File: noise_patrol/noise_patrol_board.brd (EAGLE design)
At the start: 53.5 x 57.3 mm, 25 parts, among them IC1 4511D, Q1 TIP31C, U1 OPA345NA/3K

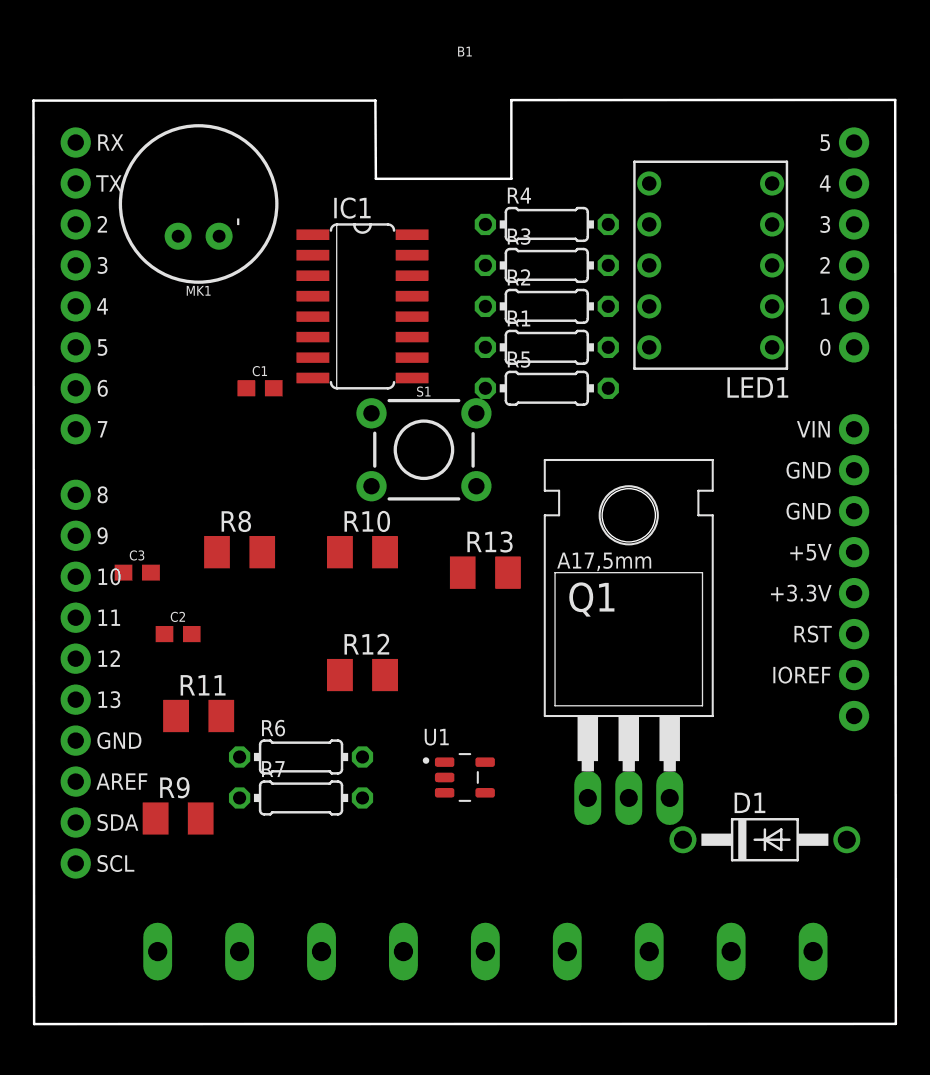
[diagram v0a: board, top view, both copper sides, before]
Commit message: Finished
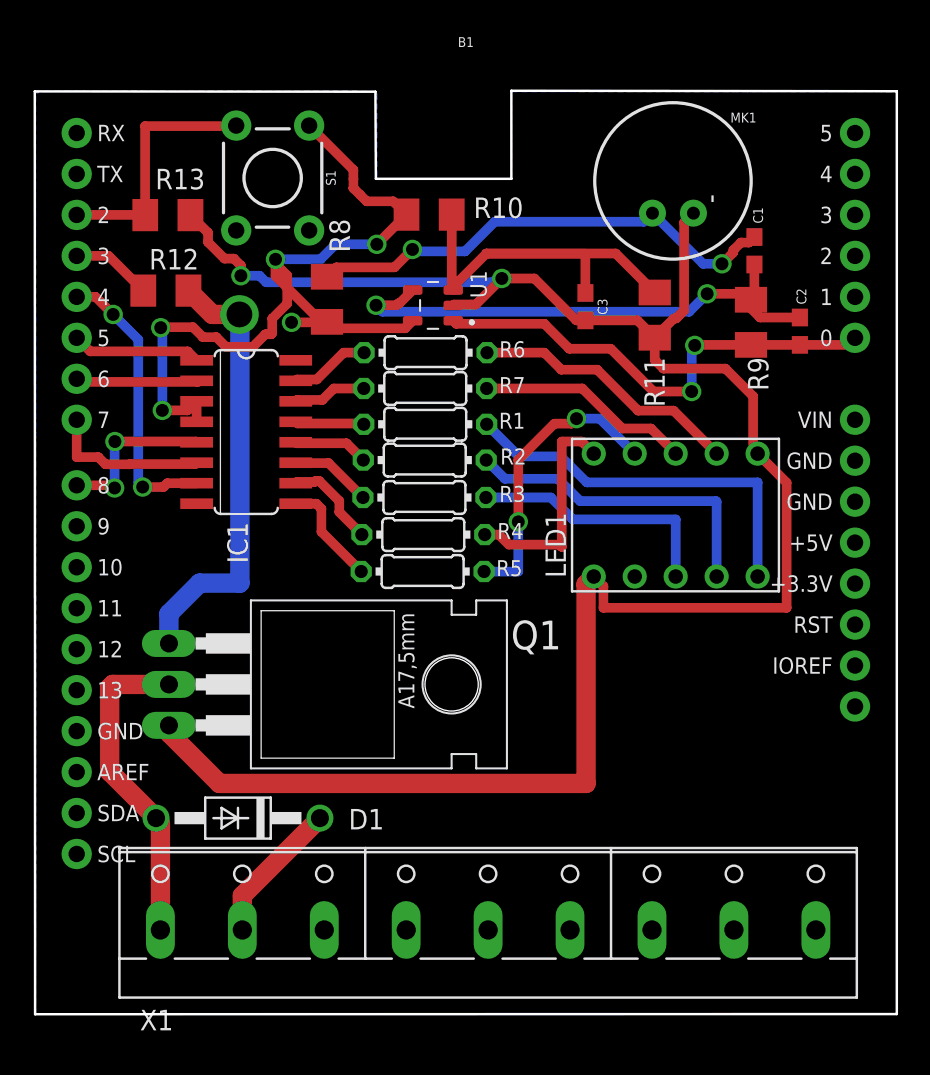
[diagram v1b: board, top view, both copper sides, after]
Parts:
- S1: value MOMENTARY-SWITCH-SPST-PTH-6.0MM -> Reset button
- moved R9 47.0 mm to (63.5, 58.7), turned to 270 degrees
- moved C2 42.9 mm to (66.5, 58.1), turned to 270 degrees
- moved R11 37.7 mm to (57.5, 59.1), turned to 270 degrees
- moved D1 32.7 mm to (31.6, 28.0), turned to 180 degrees
- moved C3 32.3 mm to (53.2, 59.7), turned to 270 degrees
- moved C1 31.8 mm to (63.7, 63.1), turned to 270 degrees
- moved R13 29.7 mm to (27.3, 65.3), turned to 180 degrees
- moved MK1 29.4 mm to (58.6, 67.5)
- moved U1 29.3 mm to (43.7, 59.8), turned to 180 degrees
- moved R12 26.8 mm to (27.2, 60.7)
- moved R7 26.5 mm to (43.3, 54.6)
- moved R6 26.2 mm to (43.3, 56.8)
- moved Q1 22.2 mm to (33.7, 36.2), turned to 270 degrees
- moved R10 21.3 mm to (43.5, 65.4)
- moved R4 20.7 mm to (43.1, 45.5)
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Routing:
- net GND: track 0.00 -> 121.9 mm, vias 0 -> 2
- net 5V: track 0.00 -> 53.8 mm, vias 0 -> 5
- net N$21: track 0.00 -> 32.8 mm, vias 0 -> 2
- net N$20: track 0.00 -> 30.3 mm, vias 0 -> 2
- net N$18: track 0.00 -> 29.7 mm, vias 0 -> 2
- net N$24: track 0.00 -> 27.7 mm
- net N$23: track 0.00 -> 27.5 mm, vias 0 -> 1
- net N$13: track 0.00 -> 24.1 mm
- net N$25: track 0.00 -> 20.1 mm
- net N$12: track 0.00 -> 20.0 mm
- net N$9: track 0.00 -> 18.2 mm, vias 0 -> 2
- net N$14: track 0.00 -> 17.6 mm, vias 0 -> 2
- net N$8: track 0.00 -> 16.8 mm
- net N$11: track 0.00 -> 15.9 mm
- net N$27: track 0.00 -> 15.4 mm
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- added copper zone on layer 16, net GND
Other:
- outline, holes or cut-outs redrawn
